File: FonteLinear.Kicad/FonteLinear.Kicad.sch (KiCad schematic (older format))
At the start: 26 parts, among them J1 Conn_01x03_Male, J2 Conn_01x02_Male, J3 Conn_01x02_Male, J4 Conn_01x02_Male, J5 Conn_01x02_Male, U1 LM317_TO39, U2 LM7805_TO220, U3 LM7815_TO220, U4 LM7915_TO220

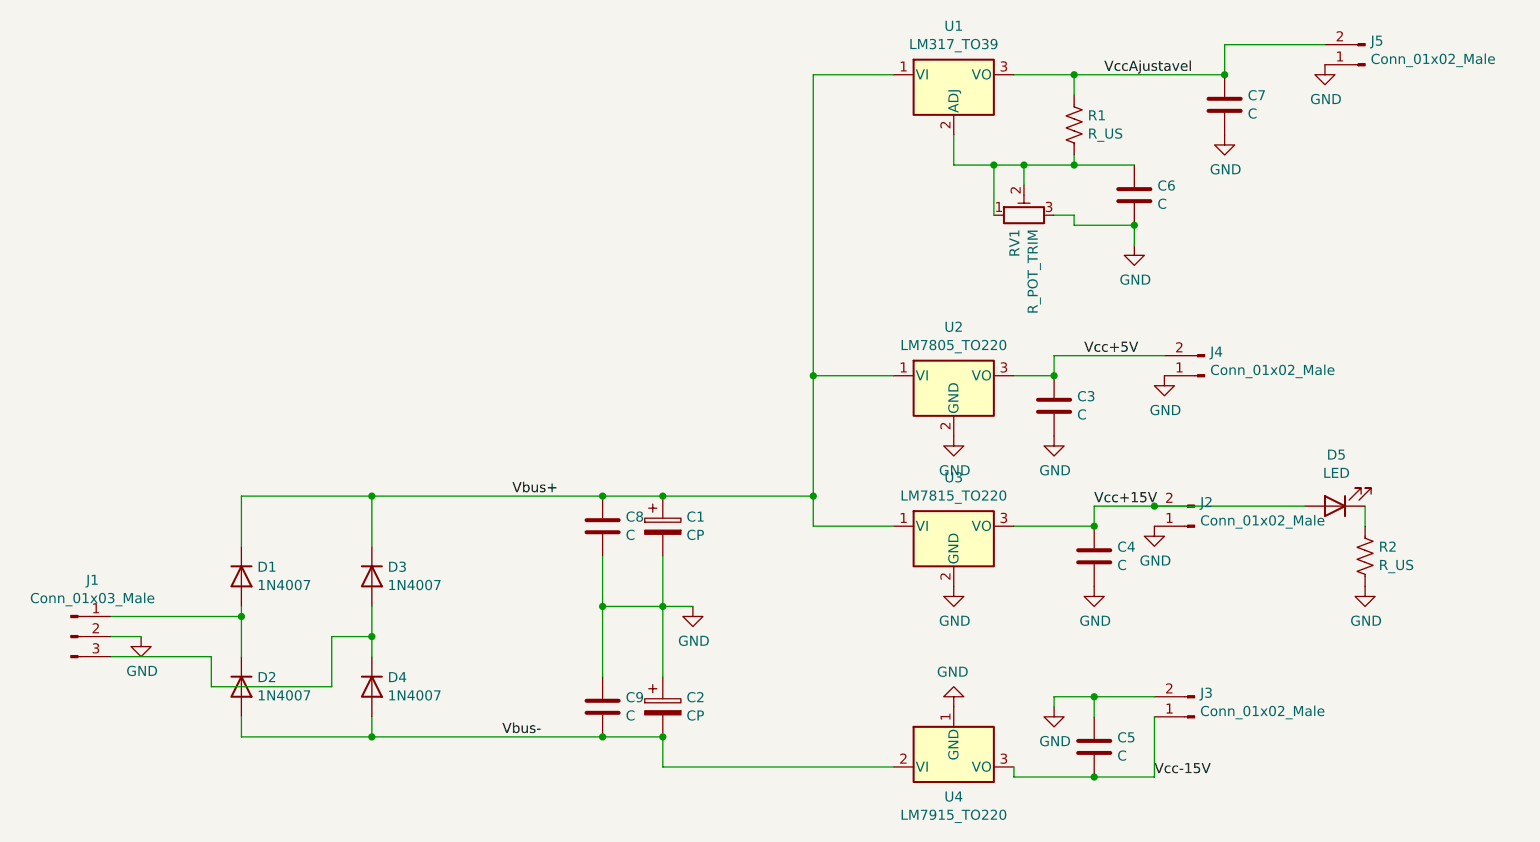
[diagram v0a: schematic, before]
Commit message: Add files via upload
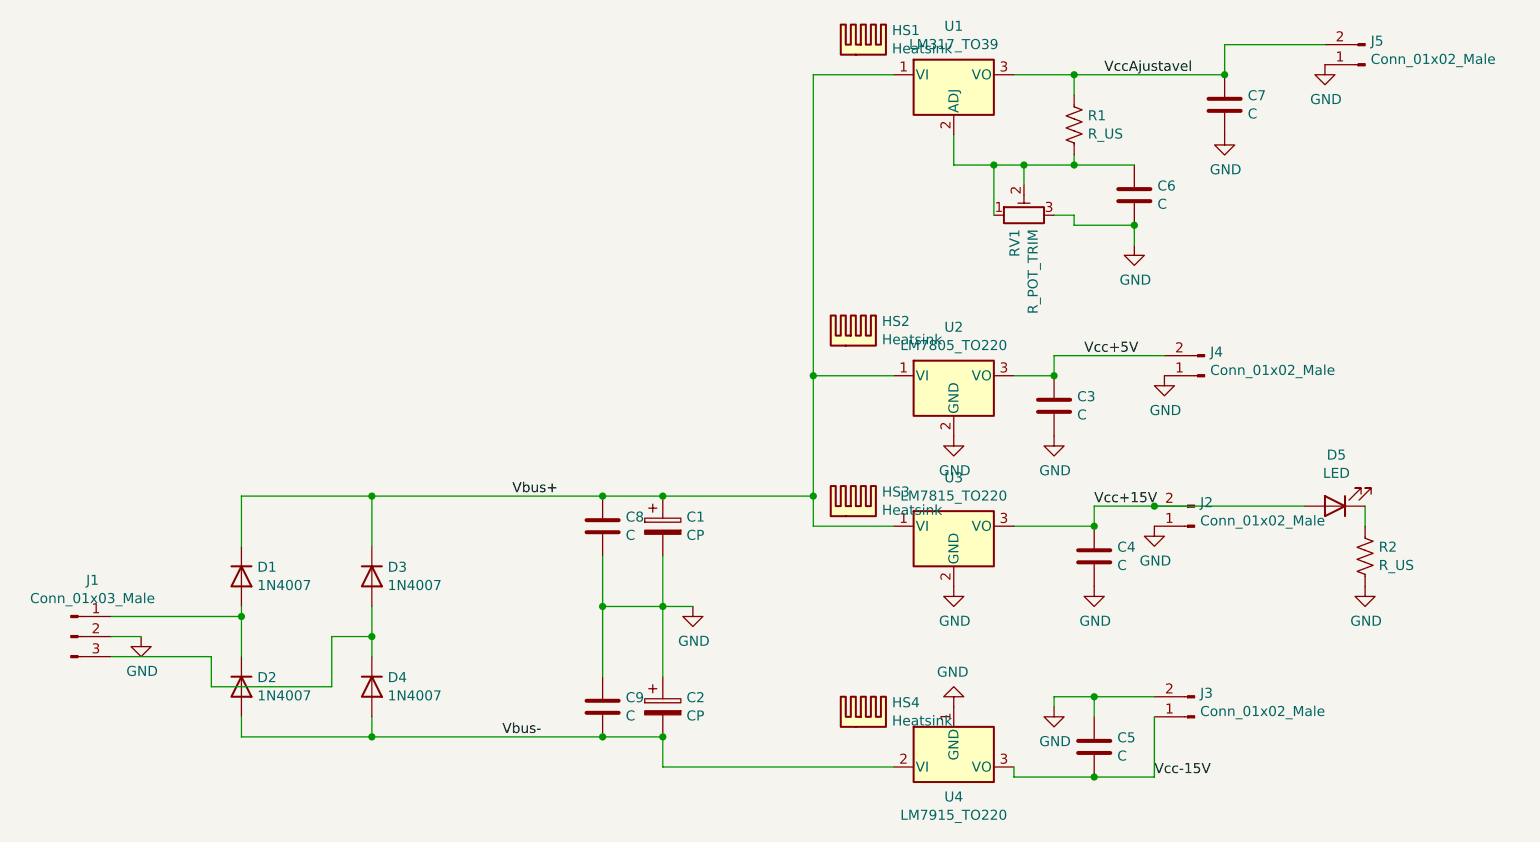
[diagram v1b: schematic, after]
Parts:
- added HS1, HS2, HS3, HS4: Heatsink, Heatsinks:Heatsink_Stonecold_HS-132_32x14mm_2xFixation1.5mm, symbol Mechanical:Heatsink
- C1, C2: footprint Capacitors_THT:CP_Radial_D16.0mm_P7.50mm -> Capacitor_THT:CP_Radial_D16.0mm_P7.50mm
- C3, C4, C5, C6, C7, C8, C9: footprint Resistors_THT:R_Axial_DIN0309_L9.0mm_D3.2mm_P5.08mm_Vertical -> Capacitors_THT:C_Disc_D5.0mm_W2.5mm_P2.50mm
- D1, D2, D3, D4: footprint Diodes_THT:D_DO-41_SOD81_P10.16mm_Horizontal -> Diode_THT:D_DO-41_SOD81_P10.16mm_Horizontal
- D5: footprint Diodes_THT:D_DO-35_SOD27_P5.08mm_Vertical_AnodeUp -> LEDs:LED_D5.0mm
- J1: footprint Pin_Headers:Pin_Header_Angled_1x03_Pitch2.54mm -> Connector_PinHeader_2.54mm:PinHeader_1x03_P2.54mm_Vertical
- J2, J3, J4, J5: footprint Pin_Headers:Pin_Header_Angled_1x02_Pitch2.54mm -> Connector_PinHeader_2.54mm:PinHeader_1x02_P2.54mm_Vertical
- R1, R2: footprint Resistors_THT:R_Axial_DIN0309_L9.0mm_D3.2mm_P5.08mm_Vertical -> Resistors_THT:R_Axial_DIN0207_L6.3mm_D2.5mm_P7.62mm_Horizontal
- RV1: footprint Potentiometers:Potentiometer_Trimmer_Vishay_43 -> Potentiometer_THT:Potentiometer_Bourns_3005_Horizontal
- U1, U2, U3, U4: footprint Power_Integrations:TO-220 -> Package_TO_SOT_THT:TO-220-3_Vertical
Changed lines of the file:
@@
 EESchema Schematic File Version 4
-EELAYER 29 0
+EELAYER 30 0
 EELAYER END
 $Descr A4 11693 8268
@@
 F 0 "C1" H 3968 4646 50  0000 L CNN
 F 1 "CP" H 3968 4555 50  0000 L CNN
-F 2 "Capacitors_THT:CP_Radial_D16.0mm_P7.50mm" H 3888 4450 50  0001 C CNN
+F 2 "Capacitor_THT:CP_Radial_D16.0mm_P7.50mm" H 3888 4450 50  0001 C CNN
 F 3 "~" H 3850 4600 50  0001 C CNN
 	1    3850 4600
@@
 F 0 "C2" H 3968 5546 50  0000 L CNN
 F 1 "CP" H 3968 5455 50  0000 L CNN
-F 2 "Capacitors_THT:CP_Radial_D16.0mm_P7.50mm" H 3888 5350 50  0001 C CNN
+F 2 "Capacitor_THT:CP_Radial_D16.0mm_P7.50mm" H 3888 5350 50  0001 C CNN
 F 3 "~" H 3850 5500 50  0001 C CNN
 	1    3850 5500
@@
 F 0 "U4" H 5300 5651 50  0000 C CNN
 F 1 "LM7915_TO220" H 5300 5560 50  0000 C CNN
-F 2 "Power_Integrations:TO-220" H 5300 5600 50  0001 C CIN
+F 2 "Package_TO_SOT_THT:TO-220-3_Vertical" H 5300 5600 50  0001 C CIN
 F 3 "http://www.fairchildsemi.com/ds/LM/LM7905.pdf" H 5300 5800 50  0001 C CNN
 	1    5300 5800
@@
 F 0 "U3" H 5300 4842 50  0000 C CNN
 F 1 "LM7815_TO220" H 5300 4751 50  0000 C CNN
-F 2 "Power_Integrations:TO-220" H 5300 4825 50  0001 C CIN
+F 2 "Package_TO_SOT_THT:TO-220-3_Vertical" H 5300 4825 50  0001 C CIN
 F 3 "http://www.fairchildsemi.com/ds/LM/LM7805.pdf" H 5300 4550 50  0001 C CNN
 	1    5300 4600
@@
 F 0 "U2" H 5300 4092 50  0000 C CNN
 F 1 "LM7805_TO220" H 5300 4001 50  0000 C CNN
-F 2 "Power_Integrations:TO-220" H 5300 4075 50  0001 C CIN
+F 2 "Package_TO_SOT_THT:TO-220-3_Vertical" H 5300 4075 50  0001 C CIN
 F 3 "http://www.fairchildsemi.com/ds/LM/LM7805.pdf" H 5300 3800 50  0001 C CNN
 	1    5300 3850
@@
 F 0 "R1" H 5968 2646 50  0000 L CNN
 F 1 "R_US" H 5968 2555 50  0000 L CNN
-F 2 "Resistors_THT:R_Axial_DIN0309_L9.0mm_D3.2mm_P5.08mm_Vertical" V 5940 2590 50  0001 C CNN
+F 2 "Resistors_THT:R_Axial_DIN0207_L6.3mm_D2.5mm_P7.62mm_Horizontal" V 5940 2590 50  0001 C CNN
 F 3 "~" H 5900 2600 50  0001 C CNN
 	1    5900 2600
@@
 F 0 "J1" H 1008 5431 50  0000 C CNN
 F 1 "Conn_01x03_Male" H 1008 5340 50  0000 C CNN
-F 2 "Pin_Headers:Pin_Header_Angled_1x03_Pitch2.54mm" H 900 5150 50  0001 C CNN
+F 2 "Connector_PinHeader_2.54mm:PinHeader_1x03_P2.54mm_Vertical" H 900 5150 50  0001 C CNN
 F 3 "~" H 900 5150 50  0001 C CNN
 	1    900  5150
@@
 F 0 "J5" H 7322 2182 50  0000 R CNN
 F 1 "Conn_01x02_Male" H 7322 2273 50  0000 R CNN
-F 2 "Pin_Headers:Pin_Header_Angled_1x02_Pitch2.54mm" H 7350 2300 50  0001 C CNN
+F 2 "Connector_PinHeader_2.54mm:PinHeader_1x02_P2.54mm_Vertical" H 7350 2300 50  0001 C CNN
 F 3 "~" H 7350 2300 50  0001 C CNN
 	1    7350 2300
@@
 F 0 "J4" H 6522 3732 50  0000 R CNN
 F 1 "Conn_01x02_Male" H 6522 3823 50  0000 R CNN
-F 2 "Pin_Headers:Pin_Header_Angled_1x02_Pitch2.54mm" H 6550 3850 50  0001 C CNN
+F 2 "Connector_PinHeader_2.54mm:PinHeader_1x02_P2.54mm_Vertical" H 6550 3850 50  0001 C CNN
 F 3 "~" H 6550 3850 50  0001 C CNN
 	1    6550 3850
@@
 F 0 "J2" H 6472 4482 50  0000 R CNN
 F 1 "Conn_01x02_Male" H 6472 4573 50  0000 R CNN
-F 2 "Pin_Headers:Pin_Header_Angled_1x02_Pitch2.54mm" H 6500 4600 50  0001 C CNN
+F 2 "Connector_PinHeader_2.54mm:PinHeader_1x02_P2.54mm_Vertical" H 6500 4600 50  0001 C CNN
 F 3 "~" H 6500 4600 50  0001 C CNN
 	1    6500 4600
@@
 F 0 "J3" H 6472 5432 50  0000 R CNN
 F 1 "Conn_01x02_Male" H 6472 5523 50  0000 R CNN
-F 2 "Pin_Headers:Pin_Header_Angled_1x02_Pitch2.54mm" H 6500 5550 50  0001 C CNN
+F 2 "Connector_PinHeader_2.54mm:PinHeader_1x02_P2.54mm_Vertical" H 6500 5550 50  0001 C CNN
 F 3 "~" H 6500 5550 50  0001 C CNN
 	1    6500 5550
@@
 F 0 "D5" H 7193 4245 50  0000 C CNN
 F 1 "LED" H 7193 4336 50  0000 C CNN
-F 2 "Diodes_THT:D_DO-35_SOD27_P5.08mm_Vertical_AnodeUp" H 7200 4500 50  0001 C CNN
+F 2 "LEDs:LED_D5.0mm" H 7200 4500 50  0001 C CNN
 F 3 "~" H 7200 4500 50  0001 C CNN
 	1    7200 4500
@@
 F 0 "R2" H 7418 4796 50  0000 L CNN
 F 1 "R_US" H 7418 4705 50  0000 L CNN
-F 2 "Resistors_THT:R_Axial_DIN0309_L9.0mm_D3.2mm_P5.08mm_Vertical" V 7390 4740 50  0001 C CNN
+F 2 "Resistors_THT:R_Axial_DIN0207_L6.3mm_D2.5mm_P7.62mm_Horizontal" V 7390 4740 50  0001 C CNN
 F 3 "~" H 7350 4750 50  0001 C CNN
 	1    7350 4750
@@
 F 0 "D1" V 1704 4929 50  0000 L CNN
 F 1 "1N4007" V 1795 4929 50  0000 L CNN
-F 2 "Diodes_THT:D_DO-41_SOD81_P10.16mm_Horizontal" H 1750 4675 50  0001 C CNN
+F 2 "Diode_THT:D_DO-41_SOD81_P10.16mm_Horizontal" H 1750 4675 50  0001 C CNN
 F 3 "http://www.vishay.com/docs/88503/1n4001.pdf" H 1750 4850 50  0001 C CNN
 	1    1750 4850
@@
 F 0 "D3" V 2354 4929 50  0000 L CNN
 F 1 "1N4007" V 2445 4929 50  0000 L CNN
-F 2 "Diodes_THT:D_DO-41_SOD81_P10.16mm_Horizontal" H 2400 4675 50  0001 C CNN
+F 2 "Diode_THT:D_DO-41_SOD81_P10.16mm_Horizontal" H 2400 4675 50  0001 C CNN
 F 3 "http://www.vishay.com/docs/88503/1n4001.pdf" H 2400 4850 50  0001 C CNN
 	1    2400 4850
@@
 F 0 "D2" V 1704 5479 50  0000 L CNN
 F 1 "1N4007" V 1795 5479 50  0000 L CNN
-F 2 "Diodes_THT:D_DO-41_SOD81_P10.16mm_Horizontal" H 1750 5225 50  0001 C CNN
+F 2 "Diode_THT:D_DO-41_SOD81_P10.16mm_Horizontal" H 1750 5225 50  0001 C CNN
 F 3 "http://www.vishay.com/docs/88503/1n4001.pdf" H 1750 5400 50  0001 C CNN
 	1    1750 5400
@@
 F 0 "D4" V 2354 5479 50  0000 L CNN
 F 1 "1N4007" V 2445 5479 50  0000 L CNN
-F 2 "Diodes_THT:D_DO-41_SOD81_P10.16mm_Horizontal" H 2400 5225 50  0001 C CNN
+F 2 "Diode_THT:D_DO-41_SOD81_P10.16mm_Horizontal" H 2400 5225 50  0001 C CNN
 F 3 "http://www.vishay.com/docs/88503/1n4001.pdf" H 2400 5400 50  0001 C CNN
 	1    2400 5400
@@
 F 0 "C6" H 6315 2996 50  0000 L CNN
 F 1 "C" H 6315 2905 50  0000 L CNN
-F 2 "Resistors_THT:R_Axial_DIN0309_L9.0mm_D3.2mm_P5.08mm_Vertical" H 6238 2800 50  0001 C CNN
+F 2 "Capacitors_THT:C_Disc_D5.0mm_W2.5mm_P2.50mm" H 6238 2800 50  0001 C CNN
 F 3 "~" H 6200 2950 50  0001 C CNN
 	1    6200 2950
@@
 F 0 "C8" H 3665 4646 50  0000 L CNN
 F 1 "C" H 3665 4555 50  0000 L CNN
-F 2 "Resistors_THT:R_Axial_DIN0309_L9.0mm_D3.2mm_P5.08mm_Vertical" H 3588 4450 50  0001 C CNN
+F 2 "Capacitors_THT:C_Disc_D5.0mm_W2.5mm_P2.50mm" H 3588 4450 50  0001 C CNN
 F 3 "~" H 3550 4600 50  0001 C CNN
 	1    3550 4600
@@
 F 0 "C9" H 3665 5546 50  0000 L CNN
 F 1 "C" H 3665 5455 50  0000 L CNN
-F 2 "Resistors_THT:R_Axial_DIN0309_L9.0mm_D3.2mm_P5.08mm_Vertical" H 3588 5350 50  0001 C CNN
+F 2 "Capacitors_THT:C_Disc_D5.0mm_W2.5mm_P2.50mm" H 3588 5350 50  0001 C CNN
 F 3 "~" H 3550 5500 50  0001 C CNN
 	1    3550 5500
@@
 F 0 "C7" H 6765 2546 50  0000 L CNN
 F 1 "C" H 6765 2455 50  0000 L CNN
-F 2 "Resistors_THT:R_Axial_DIN0309_L9.0mm_D3.2mm_P5.08mm_Vertical" H 6688 2350 50  0001 C CNN
+F 2 "Capacitors_THT:C_Disc_D5.0mm_W2.5mm_P2.50mm" H 6688 2350 50  0001 C CNN
 F 3 "~" H 6650 2500 50  0001 C CNN
 	1    6650 2500
@@
 F 0 "C3" H 5915 4046 50  0000 L CNN
 F 1 "C" H 5915 3955 50  0000 L CNN
-F 2 "Resistors_THT:R_Axial_DIN0309_L9.0mm_D3.2mm_P5.08mm_Vertical" H 5838 3850 50  0001 C CNN
+F 2 "Capacitors_THT:C_Disc_D5.0mm_W2.5mm_P2.50mm" H 5838 3850 50  0001 C CNN
 F 3 "~" H 5800 4000 50  0001 C CNN
 	1    5800 4000
@@
 F 0 "C4" H 6115 4796 50  0000 L CNN
 F 1 "C" H 6115 4705 50  0000 L CNN
-F 2 "Resistors_THT:R_Axial_DIN0309_L9.0mm_D3.2mm_P5.08mm_Vertical" H 6038 4600 50  0001 C CNN
+F 2 "Capacitors_THT:C_Disc_D5.0mm_W2.5mm_P2.50mm" H 6038 4600 50  0001 C CNN
 F 3 "~" H 6000 4750 50  0001 C CNN
 	1    6000 4750
@@
 F 0 "C5" H 6115 5746 50  0000 L CNN
 F 1 "C" H 6115 5655 50  0000 L CNN
-F 2 "Resistors_THT:R_Axial_DIN0309_L9.0mm_D3.2mm_P5.08mm_Vertical" H 6038 5550 50  0001 C CNN
+F 2 "Capacitors_THT:C_Disc_D5.0mm_W2.5mm_P2.50mm" H 6038 5550 50  0001 C CNN
 F 3 "~" H 6000 5700 50  0001 C CNN
 	1    6000 5700
@@
 F 0 "U1" H 5300 2592 50  0000 C CNN
 F 1 "LM317_TO39" H 5300 2501 50  0000 C CNN
-F 2 "Power_Integrations:TO-220" H 5300 2575 50  0001 C CIN
+F 2 "Package_TO_SOT_THT:TO-220-3_Vertical" H 5300 2575 50  0001 C CIN
 F 3 "http://www.ti.com/lit/ds/symlink/lm317.pdf" H 5300 2350 50  0001 C CNN
 	1    5300 2350
@@
 F 0 "RV1" H 5580 3096 50  0000 R CNN
 F 1 "R_POT_TRIM" H 5580 3005 50  0000 R CNN
-F 2 "Potentiometers:Potentiometer_Trimmer_Vishay_43" H 5650 3050 50  0001 C CNN
+F 2 "Potentiometer_THT:Potentiometer_Bourns_3005_Horizontal" H 5650 3050 50  0001 C CNN
 F 3 "~" H 5650 3050 50  0001 C CNN
 	1    5650 3050
@@
 	5900 3100 6200 3100
 Connection ~ 6200 3100
+$Comp
+L Mechanical:Heatsink HS4
+U 1 1 5F49FC1F
+P 4850 5600
+F 0 "HS4" H 4992 5721 50  0000 L CNN
+F 1 "Heatsink" H 4992 5630 50  0000 L CNN
+F 2 "Heatsinks:Heatsink_Stonecold_HS-132_32x14mm_2xFixation1.5mm" H 4862 5600 50  0001 C CNN
+F 3 "~" H 4862 5600 50  0001 C CNN
+	1    4850 5600
+	1    0    0    -1
+$EndComp
+$Comp
+L Mechanical:Heatsink HS3
+U 1 1 5F4A812D
+P 4800 4550
+F 0 "HS3" H 4942 4671 50  0000 L CNN
+F 1 "Heatsink" H 4942 4580 50  0000 L CNN
+F 2 "Heatsinks:Heatsink_Stonecold_HS-132_32x14mm_2xFixation1.5mm" H 4812 4550 50  0001 C CNN
+F 3 "~" H 4812 4550 50  0001 C CNN
+	1    4800 4550
+	1    0    0    -1
+$EndComp
+$Comp
+L Mechanical:Heatsink HS2
+U 1 1 5F4A89E3
+P 4800 3700
+F 0 "HS2" H 4942 3821 50  0000 L CNN
+F 1 "Heatsink" H 4942 3730 50  0000 L CNN
+F 2 "Heatsinks:Heatsink_Stonecold_HS-132_32x14mm_2xFixation1.5mm" H 4812 3700 50  0001 C CNN
+F 3 "~" H 4812 3700 50  0001 C CNN
+	1    4800 3700
+	1    0    0    -1
+$EndComp
+$Comp
+L Mechanical:Heatsink HS1
+U 1 1 5F4A92FA
+P 4850 2250
+F 0 "HS1" H 4992 2371 50  0000 L CNN
+F 1 "Heatsink" H 4992 2280 50  0000 L CNN
+F 2 "Heatsinks:Heatsink_Stonecold_HS-132_32x14mm_2xFixation1.5mm" H 4862 2250 50  0001 C CNN
+F 3 "~" H 4862 2250 50  0001 C CNN
+	1    4850 2250
+	1    0    0    -1
+$EndComp
 $EndSCHEMATC
